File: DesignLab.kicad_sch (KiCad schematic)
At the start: 32 parts, among them Y1 LFXTAL003000

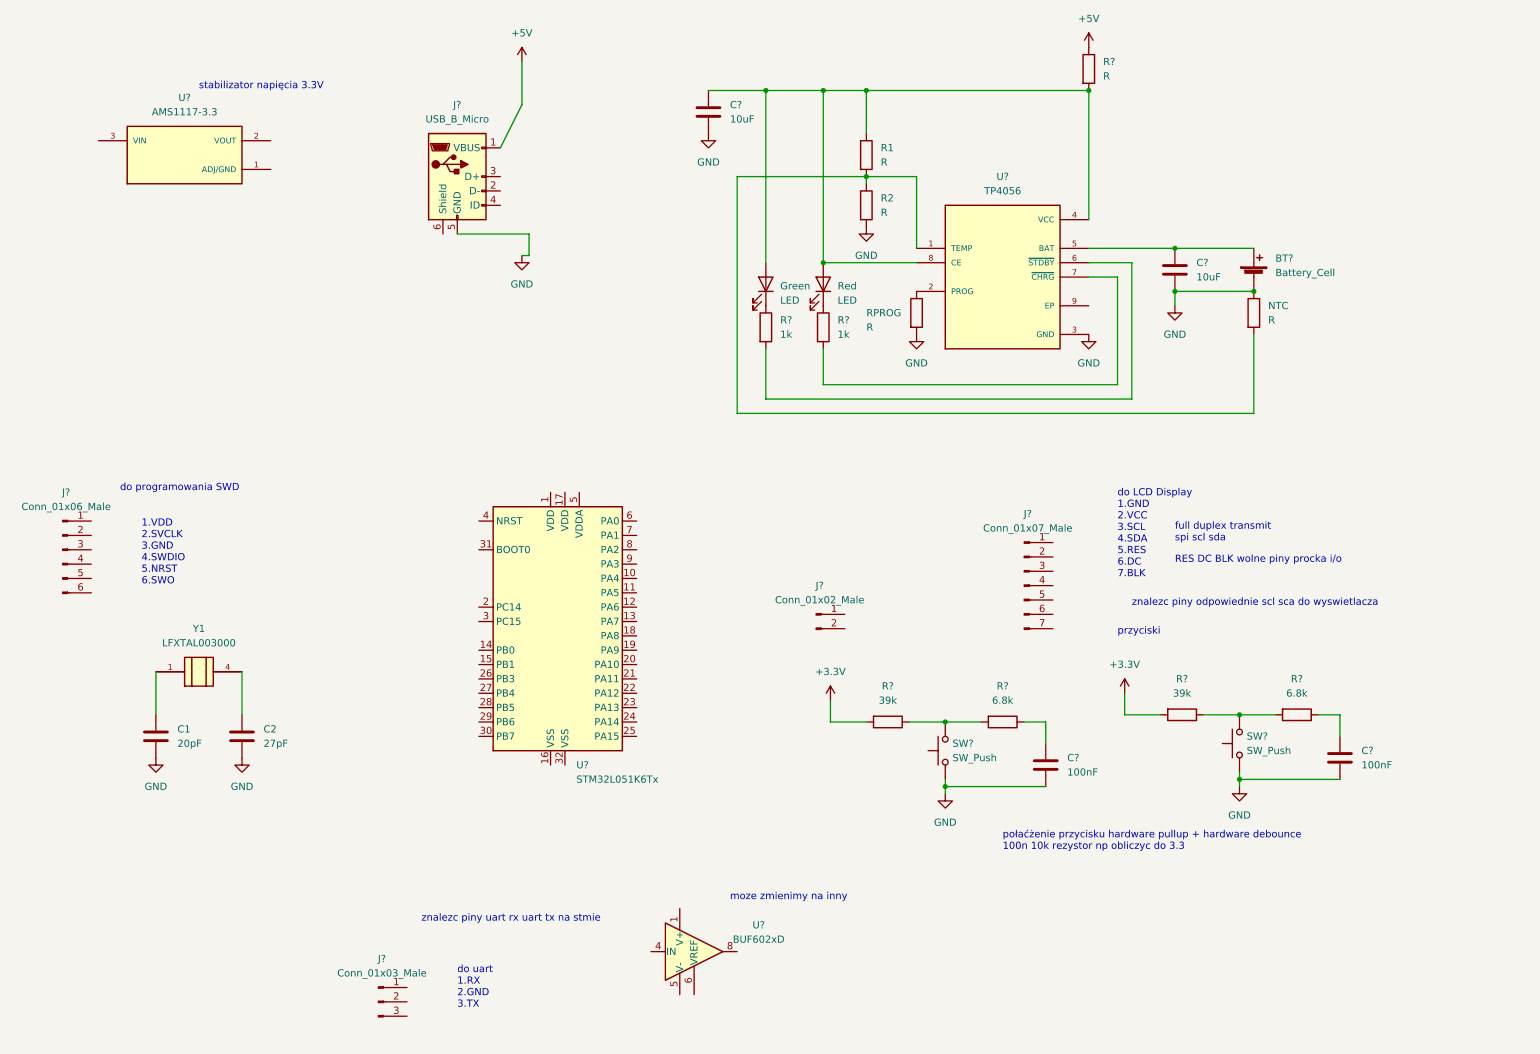
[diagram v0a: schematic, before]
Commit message: v0.2 06.12.2022 MM
Completed schematic file
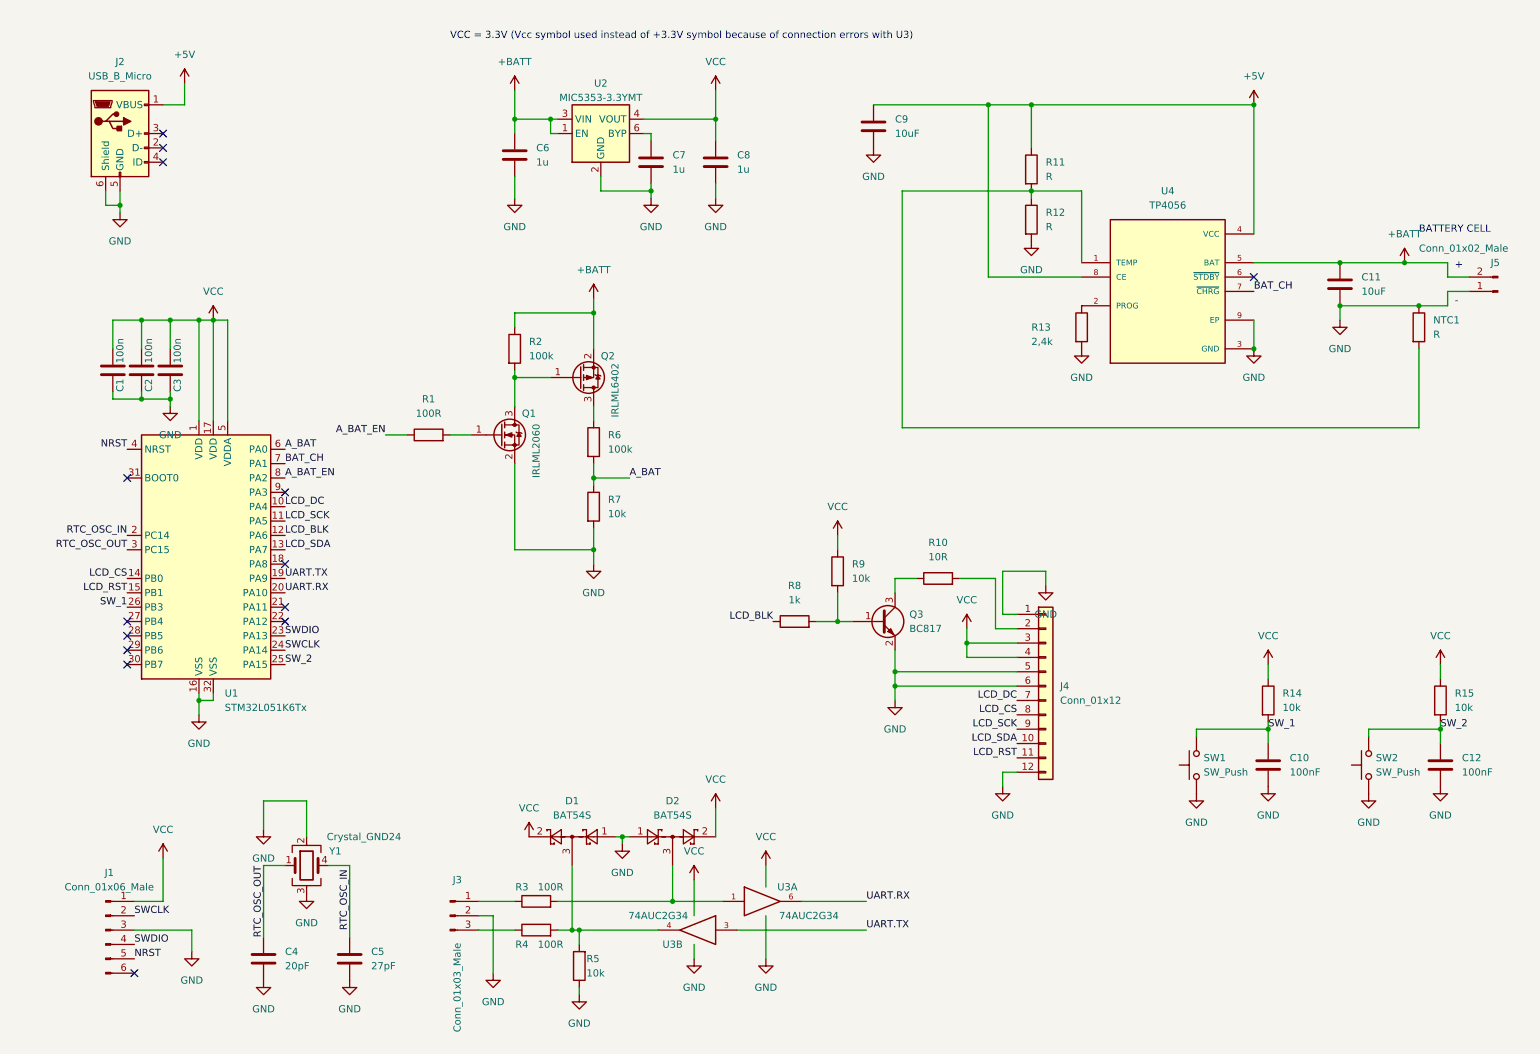
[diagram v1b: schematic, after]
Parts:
- removed BT?: Battery_Cell, symbol Device:Battery_Cell
- removed C?: 100nF, symbol Device:C
- removed Green, Red: LED, symbol Device:LED
- removed J?: Conn_01x07_Male, symbol Connector:Conn_01x07_Male
- removed R?: R, symbol Device:R
- removed R? (x2): 6.8k, symbol Device:R
- removed R?: 39k, symbol Device:R
- removed R? (x2): 1k, symbol Device:R
- removed SW?: SW_Push, symbol Switch:SW_Push
- removed U?: TP4056, SOP127P600X175-9N, symbol TP4056:TP4056
- removed U?: AMS1117-3.3, SOT229P700X180-4N, symbol AMS1117-3.3:AMS1117-3.3
- removed U?: BUF602xD, Package_SO:SOIC-8_3.9x4.9mm_P1.27mm, symbol Amplifier_Buffer:BUF602xD
- removed Y1: LFXTAL003000, XTAL_LFXTAL003000, symbol LFXTAL003000:LFXTAL003000
- added C1, C2, C3: 100n, Capacitor_SMD:C_0603_1608Metric_Pad1.08x0.95mm_HandSolder, symbol Device:C
- added C12: 100nF, Capacitor_SMD:C_0603_1608Metric_Pad1.08x0.95mm_HandSolder, symbol Device:C
- added C6, C7, C8: 1u, Capacitor_SMD:C_0805_2012Metric_Pad1.18x1.45mm_HandSolder, symbol Device:C
- added D1, D2: BAT54S, Package_TO_SOT_SMD:SOT-23, symbol Diode:BAT54S
- added J4: Conn_01x12, Connector:Flex_Tape_12x0.635, symbol Connector_Generic:Conn_01x12
- added Q1: IRLML2060, Package_TO_SOT_SMD:SOT-23, symbol Transistor_FET:IRLML2060
- added Q2: IRLML6402, Package_TO_SOT_SMD:SOT-23, symbol Transistor_FET:IRLML6402
- added Q3: BC817, Package_TO_SOT_SMD:SOT-23, symbol Transistor_BJT:BC817
- added R1, R3, R4: 100R, Resistor_SMD:R_0603_1608Metric_Pad0.98x0.95mm_HandSolder, symbol Device:R
- added R10: 10R, Resistor_SMD:R_0603_1608Metric_Pad0.98x0.95mm_HandSolder, symbol Device:R
- added R15, R5, R7, R9: 10k, Resistor_SMD:R_0603_1608Metric_Pad0.98x0.95mm_HandSolder, symbol Device:R
- added R2, R6: 100k, Resistor_SMD:R_0603_1608Metric_Pad0.98x0.95mm_HandSolder, symbol Device:R
- added R8: 1k, Resistor_SMD:R_0603_1608Metric_Pad0.98x0.95mm_HandSolder, symbol Device:R
- added SW2: SW_Push, Button_Switch_SMD:SW_SPST_B3U-3000P-B, symbol Switch:SW_Push
- added U2: MIC5353-3.3YMT, Package_DFN_QFN:MLF-6-1EP_1.6x1.6mm_P0.5mm_EP0.5x1.26mm, symbol Regulator_Linear:MIC5353-3.3YMT
- added U3: 74AUC2G34, Package_TO_SOT_SMD:SOT-23-6_Handsoldering, symbol 74xGxx:74AUC2G34
- added U4: TP4056, Package_SO:HSOP-8-1EP_3.9x4.9mm_P1.27mm_EP2.41x3.1mm, symbol Battery_Management:TP4056
- added Y1: Crystal_GND24, Crystal:Crystal_SMD_Abracon_ABS25-4Pin_8.0x3.8mm, symbol Device:Crystal_GND23
- C10: renamed from C?; footprint (none) -> Capacitor_SMD:C_0603_1608Metric_Pad1.08x0.95mm_HandSolder
- C11, C9: renamed from C?; footprint (none) -> Capacitor_SMD:C_1206_3216Metric_Pad1.33x1.80mm_HandSolder
- C4: renamed from C1; footprint (none) -> Capacitor_SMD:C_0603_1608Metric_Pad1.08x0.95mm_HandSolder
- C5: renamed from C2; footprint (none) -> Capacitor_SMD:C_0603_1608Metric_Pad1.08x0.95mm_HandSolder
- J1: renamed from J?; footprint (none) -> Connector_PinHeader_2.54mm:PinHeader_1x06_P2.54mm_Vertical
- J2: renamed from J?; footprint (none) -> Connector_USB:USB_Micro-B_Amphenol_10104110_Horizontal
- J3: renamed from J?; footprint (none) -> Connector_PinHeader_2.54mm:PinHeader_1x03_P2.54mm_Vertical
- J5: renamed from J?; footprint (none) -> Connector_PinHeader_2.54mm:PinHeader_1x02_P2.54mm_Vertical
- NTC1: renamed from NTC; footprint (none) -> Connector_Wire:SolderWire-0.5sqmm_1x02_P4.6mm_D0.9mm_OD2.1mm
- R11: renamed from R1; footprint (none) -> Resistor_SMD:R_0603_1608Metric_Pad0.98x0.95mm_HandSolder
- R12: renamed from R2; footprint (none) -> Resistor_SMD:R_0603_1608Metric_Pad0.98x0.95mm_HandSolder
- R13: renamed from RPROG; value R -> 2,4k; footprint (none) -> Resistor_SMD:R_0603_1608Metric_Pad0.98x0.95mm_HandSolder
- R14: renamed from R?; value 39k -> 10k; footprint (none) -> Resistor_SMD:R_0603_1608Metric_Pad0.98x0.95mm_HandSolder
- SW1: renamed from SW?; footprint (none) -> Button_Switch_SMD:SW_SPST_B3U-3000P-B
- gave numbers to parts that had none: 1
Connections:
- net +3.3V is gone; now on net SW_1: R14.2
- net +5V: now also C9.1, R11.1, U4.4 (VCC), U4.8 (CE)
- net GND: now also J1.3 (Pin_3), J2.6 (Shield), J3.2 (Pin_2), J5.1 (Pin_1), U1.16 (VSS), U1.32 (VSS), C1.2, C12.2, C2.2, C3.2, C6.2, C7.2, C8.2, D1.1, D2.1, J4.1 (Pin_1), J4.12 (Pin_12), J4.5 (Pin_5), J4.6 (Pin_6), Q1.2 (S), Q3.2 (E), R5.1, R7.2, SW2.1, U2.2 (GND), U2.7 (GND), U3.2 (GND), U3.2 (GND), U4.3 (GND), U4.9 (EP), Y1.2, Y1.3
- net at NTC1.2, R11.2, R12.1: now also U4.1 (TEMP)
- net at R13.1: now also U4.2 (PROG)
- net +BATT: now reaches C11.1
- net +BATT: now also J5.2 (Pin_2), C6.1, Q2.2 (S), R2.1, U2.1 (EN), U2.3 (VIN), U4.5 (BAT)
- net SW_1: now reaches SW1.2
- net SW_1: now also C10.1, U1.26 (PB3); no longer R14.1
- net RTC_OSC_OUT: now reaches C4.1
- net RTC_OSC_OUT: now also U1.3 (PC15), Y1.1
- net RTC_OSC_IN: now reaches C5.1
- net RTC_OSC_IN: now also U1.2 (PC14), Y1.4
- net at J3.1 (Pin_1): now also R3.1
- net at J3.3 (Pin_3): now also R4.1
- net VCC: now reaches U1.1 (VDD)
- net VCC: now also J1.1 (Pin_1), R14.1, U1.17 (VDD), U1.5 (VDDA), C1.1, C2.1, C3.1, C8.1, D1.2, D2.2, J4.3 (Pin_3), J4.4 (Pin_4), R15.1, R9.1, U2.4 (VOUT), U3.5 (VCC), U3.5 (VCC)
- net LCD_DC: now reaches U1.10 (PA4)
- net LCD_DC: now also J4.7 (Pin_7)
- net LCD_SCK: now reaches U1.11 (PA5)
- net LCD_SCK: now also J4.9 (Pin_9)
- net LCD_BLK: now reaches U1.12 (PA6)
- net LCD_BLK: now also R8.1
- net LCD_SDA: now reaches U1.13 (PA7)
- net LCD_SDA: now also J4.10 (Pin_10)
- net LCD_CS: now reaches U1.14 (PB0)
- net LCD_CS: now also J4.8 (Pin_8)
- net LCD_RST: now reaches U1.15 (PB1)
- net LCD_RST: now also J4.11 (Pin_11)
- net UART.TX: now reaches U1.19 (PA9)
- net UART.TX: now also U3.3
- net UART.RX: now reaches U1.20 (PA10)
- net UART.RX: now also U3.6
- net SWDIO: now reaches U1.23 (PA13)
- net SWDIO: now also J1.4 (Pin_4)
- net SWCLK: now reaches U1.24 (PA14)
- net SWCLK: now also J1.2 (Pin_2)
- net SW_2: now reaches U1.25 (PA15)
- net SW_2: now also C12.1, R15.2, SW2.2
- net NRST: now reaches U1.4 (NRST)
- net NRST: now also J1.5 (Pin_5)
- net A_BAT: now reaches U1.6 (PA0)
- net A_BAT: now also R6.2, R7.1
- net BAT_CH: now reaches U1.7 (PA1)
- net BAT_CH: now also U4.7 (~{CHRG})
- net A_BAT_EN: now reaches U1.8 (PA2)
- net A_BAT_EN: now also R1.1
- new net: Q1.1 (G), R1.2
- new net: Q1.3 (D), Q2.1 (G), R2.2
- new net: D1.3, R4.2, R5.2, U3.4
- new net: Q2.3 (D), R6.1
- new net: D2.3, R3.2, U3.1
- new net: Q3.3 (C), R10.1
- new net: J4.2 (Pin_2), R10.2
- new net: Q3.1 (B), R8.2, R9.2
- new net: C7.1, U2.6 (BYP)
- no-connect marks 0 -> 14
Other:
- note added: "+"
- note added: "-"
- note added: "BATTERY CELL"
- note added: "VCC = 3.3V (Vcc symbol used instead of +3.3V symbol because of connection errors with U3)"
- note removed: "1.VDD 2.SVCLK 3.GND 4.SWDIO 5.NRST 6.SWO"
- note removed: "RES DC BLK wolne piny procka i/o"
- note removed: "do LCD Display 1.GND 2.VCC 3.SCL 4.SDA 5.RES 6.DC 7.BLK"
- note removed: "do programowania SWD"
- note removed: "do uart 1.RX 2.GND 3.TX"
- note removed: "full duplex transmit spi scl sda"
- note removed: "moze zmienimy na inny"
- note removed: "połaćżenie przycisku hardware pullup + hardware debounce 100n 10k rezystor np obliczyc do 3.3"
- note removed: "przyciski"
- note removed: "stabilizator napięcia 3.3V"
- note removed: "znalezc piny odpowiednie scl sca do wyswietlacza"
- note removed: "znalezc piny uart rx uart tx na stmie"
- moved on the sheet: C10, C11, C4, C5, C9, J1, J2, J3, J5, NTC1, R11, R12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
